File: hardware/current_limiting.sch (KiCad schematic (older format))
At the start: 7 parts, among them U7 TPS2557

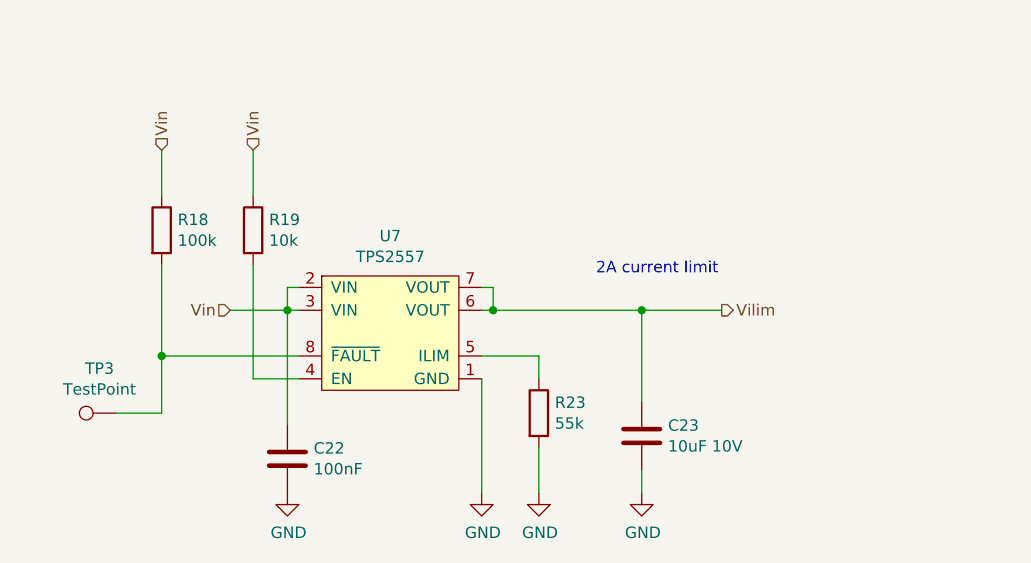
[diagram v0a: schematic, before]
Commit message: Layout partially done before change of plans
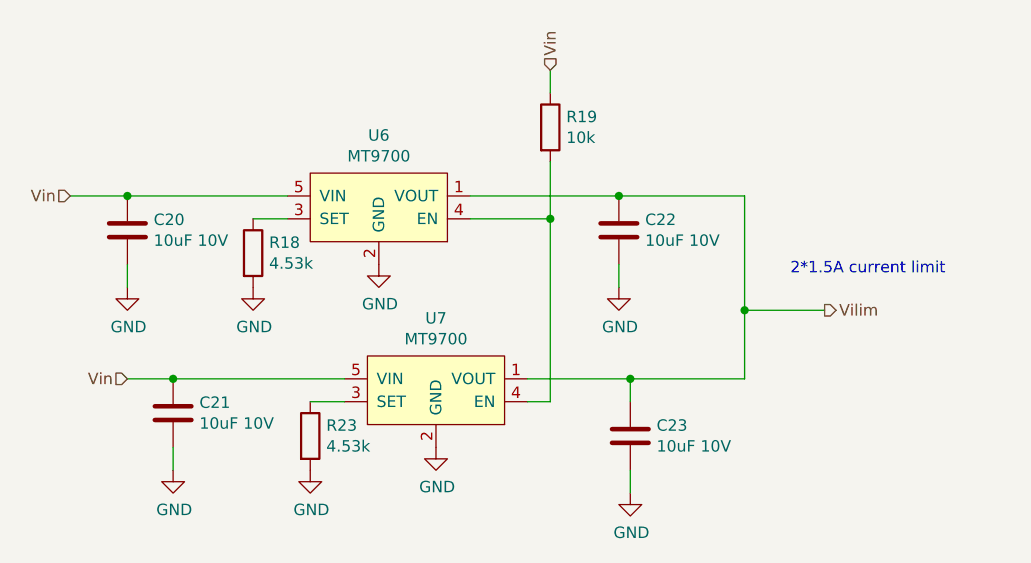
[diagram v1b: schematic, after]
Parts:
- removed TP3: TestPoint, symbol Connector:TestPoint
- removed U7: TPS2557, symbol pi-supercap-ups:TPS2557
- added C20, C21: 10uF 10V, Capacitor_SMD:C_0603_1608Metric_Pad1.05x0.95mm_HandSolder, symbol Device:C
- added U6, U7: MT9700, Package_TO_SOT_SMD:SOT-23-5_HandSoldering, symbol pi-supercap-ups:MT9700
- C22: value 100nF -> 10uF 10V; footprint (none) -> Capacitor_SMD:C_0603_1608Metric_Pad1.05x0.95mm_HandSolder
- C23: footprint (none) -> Capacitor_SMD:C_0603_1608Metric_Pad1.05x0.95mm_HandSolder
- R18: value 100k -> 4.53k
- R23: value 55k -> 4.53k
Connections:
- net GND: now also R18.2, C20.2, C21.2, U6.2 (GND), U7.2 (GND)
- net Vilim: now also C22.1, U6.1 (VOUT), U7.1 (VOUT)
- net Vin: now also C20.1, C21.1, U6.5 (VIN), U7.5 (VIN); no longer C22.1, R18.1
- net at R19.2: now also U6.4 (EN), U7.4 (EN)
- net at R23.1: now also U7.3 (SET)
- new net: R18.1, U6.3 (SET)
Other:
- note added: "2*1.5A current limit"
- note removed: "2A current limit"
- moved on the sheet: C23, R19, R23
